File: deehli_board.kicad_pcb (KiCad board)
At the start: 2 copper layers, 84 x 51 mm, 46 parts, among them J1 Servo_Out, J2 PWM_In, J3 Vcc_Out, J4 ZDT_Pins, J5 CAN_Ext, J6 Board_IO, J7 ZDT_Connector, SW1 SW_DPDT_x2, U1 APE1707M-50-HF, U2 LM2576HVT-5, U3 LM2576HVT-5, U4 LM2576HVT-15, U5 LD1117S33TR_SOT223, U6 LM2576HVT-15

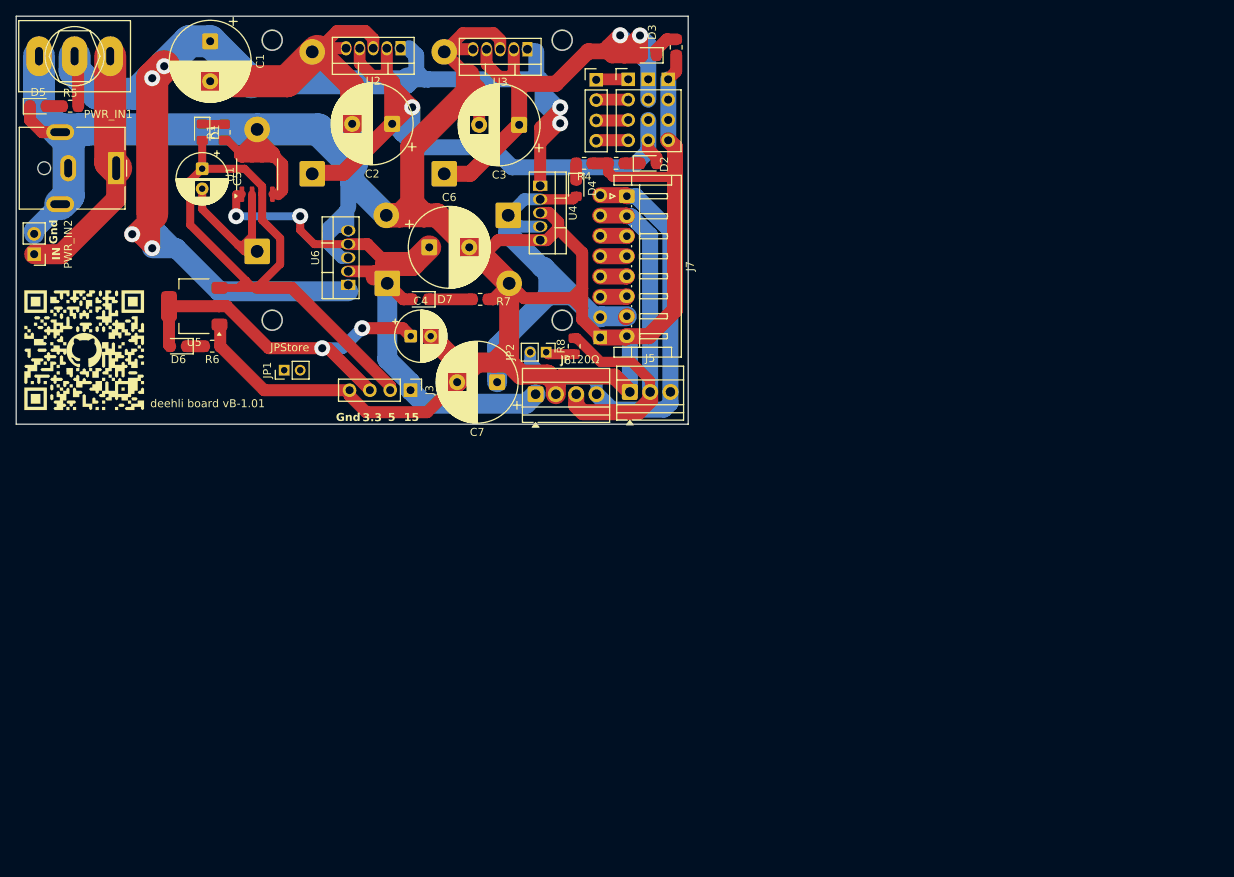
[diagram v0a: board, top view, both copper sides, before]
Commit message: VB-1.02
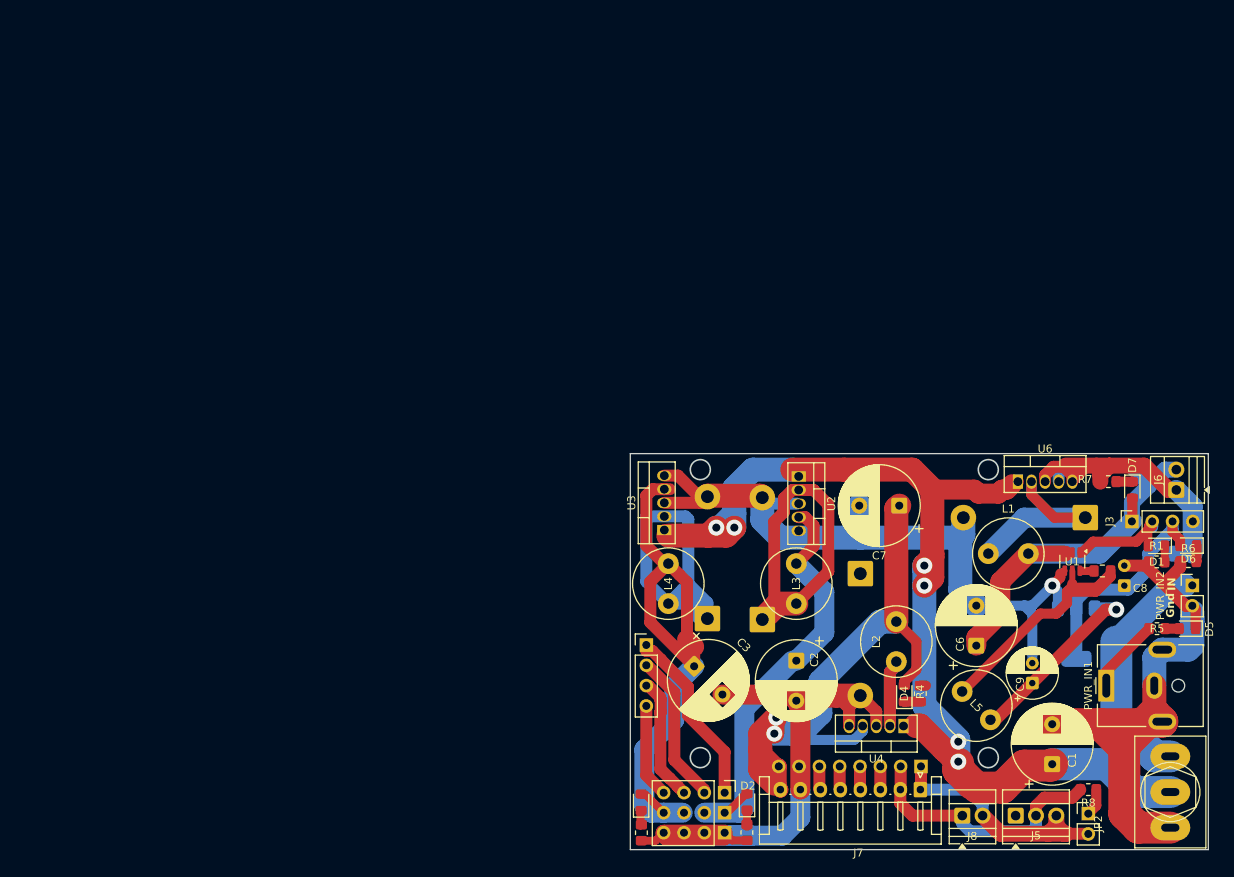
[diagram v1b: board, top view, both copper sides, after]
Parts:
- removed C5: Cpol 200uF, Capacitor_THT:CP_Radial_D6.3mm_P2.50mm
- removed D12: 1N5822, Diode_THT:D_DO-201AD_P15.24mm_Horizontal
- removed JP1: Jumper_Dummy, Connector_PinHeader_2.00mm:PinHeader_1x02_P2.00mm_Vertical
- added C8: 100nF, Capacitor_SMD:C_0805_2012Metric_Pad1.18x1.45mm_HandSolder, F.Cu at (163.8, 105.3)
- added C9: Cpol 2x22uF, Capacitor_THT:CP_Radial_D6.3mm_P2.50mm, F.Cu at (155.0, 119.4)
- added J8: BoardCAN, TerminalBlock:TerminalBlock_Xinya_XY308-2.54-2P_1x02_P2.54mm_Horizontal, F.Cu at (146.3, 135.9)
- added L1: 100u, Inductor_THT:L_Radial_D8.7mm_P5.00mm_Fastron_07HCP, F.Cu at (149.5, 103.2)
- added L2: 100u, Inductor_THT:L_Radial_D8.7mm_P5.00mm_Fastron_07HCP, F.Cu at (138.0, 116.7)
- added L3: 100u, Inductor_THT:L_Radial_D8.7mm_P5.00mm_Fastron_07HCP, F.Cu at (125.5, 109.4)
- added L4: 100u, Inductor_THT:L_Radial_D8.7mm_P5.00mm_Fastron_07HCP, F.Cu at (109.5, 109.4)
- added L5: 4.7u, Inductor_THT:L_Radial_D8.7mm_P5.00mm_Fastron_07HCP, F.Cu at (146.2, 120.4)
- C4, G***, U5: moved to B.Cu
- J3: footprint Connector_PinHeader_2.54mm:PinHeader_1x04_P2.54mm_Vertical -> Connector_PinSocket_2.54mm:PinSocket_1x04_P2.54mm_Vertical
- J4: footprint Connector_PinHeader_2.54mm:PinHeader_1x08_P2.54mm_Horizontal -> Connector_PinSocket_2.54mm:PinSocket_1x08_P2.54mm_Horizontal
- J6: value Board_IO -> BoardPWR; footprint TerminalBlock:TerminalBlock_Xinya_XY308-2.54-4P_1x04_P2.54mm_Horizontal -> TerminalBlock:TerminalBlock_Xinya_XY308-2.54-2P_1x02_P2.54mm_Horizontal
- JP2: footprint Connector_PinHeader_2.00mm:PinHeader_1x02_P2.00mm_Vertical -> Connector_PinHeader_2.54mm:PinHeader_1x02_P2.54mm_Vertical
- R5: value 15k -> 50k
- U1: value APE1707M-50-HF -> AP63205WU; footprint Package_SO:SOIC-8_3.9x4.9mm_P1.27mm -> Package_TO_SOT_SMD:TSOT-23-6
- moved SW1 165.0 mm to (172.3, 133.0), turned to 90 degrees
- moved D5 157.8 mm to (174.4, 112.6), turned to 180 degrees
- moved R5 150.7 mm to (170.6, 112.6), turned to 180 degrees
- moved PWR_IN2 150.6 mm to (175.0, 107.2), turned to 0 degrees
- moved PWR_IN1 139.6 mm to (164.3, 119.7), turned to 90 degrees
- moved C1 138.7 mm to (157.5, 129.5), turned to 90 degrees
- moved G*** 137.4 mm to (164.0, 129.0), turned to 180 degrees
- moved D1 130.0 mm to (170.5, 102.2), turned to 180 degrees
- moved D6 128.7 mm to (174.5, 102.2)
- moved R1 128.3 mm to (170.6, 104.2), turned to 0 degrees
- moved R6 124.9 mm to (174.5, 104.2), turned to 0 degrees
- moved U5 117.6 mm to (160.5, 113.2), turned to -90 degrees
- moved U1 112.8 mm to (160.0, 104.2), turned to -90 degrees
- moved R2 98.3 mm to (106.1, 138.1)
- moved C4 94.5 mm to (166.5, 107.2), turned to 90 degrees
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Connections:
- D10 pad 1: 5V_Servo12 -> Net-(D10-K)
- D11 pad 1: 15V_Other -> Net-(D11-K)
- D8 pad 1: 15V_ZDT -> Net-(D8-K)
- D9 pad 1: 5V_Servo34 -> Net-(D9-K)
- J1 pad 5: 5V_Servo12 -> 5V_Servo34
- J1 pad 6: 5V_Servo12 -> 5V_Servo34
- J1 pad 7: 5V_Servo34 -> 5V_Servo12
- J1 pad 8: 5V_Servo34 -> 5V_Servo12
- J4 pad 1: GND -> CAN_L
- J4 pad 2: 15V_ZDT -> CAN_H
- J4 pad 7: CAN_H -> GND
- J4 pad 8: CAN_L -> 15V_ZDT
- J6 pad 1: 15V_Other -> GND
- J6 pad 2: GND -> 15V_Other
- J7 pad 3: Net-(J4-Pin_6) -> Net-(J4-Pin_3)
- J7 pad 4: Net-(J4-Pin_5) -> Net-(J4-Pin_4)
- J7 pad 5: Net-(J4-Pin_4) -> Net-(J4-Pin_5)
- J7 pad 6: Net-(J4-Pin_3) -> Net-(J4-Pin_6)
- J7 pad 7: 15V_ZDT -> GND
- J7 pad 8: GND -> 15V_ZDT
- R5 pad 2: Net-(SW1A-B) -> Net-(PWR_IN2-Pin_1)
- U1 pad 1: 15V_Other -> 5V_Other
- U1 pad 2: Net-(D12-K) -> 15V_Other
- U1 pad 3: 5V_Other -> 15V_Other
- U1 pad 5: GND -> Net-(U1-SW)
- U1 pad 6: GND -> Net-(U1-BST)
- U2 pad 2: 5V_Servo34 -> Net-(D9-K)
- U3 pad 2: 5V_Servo12 -> Net-(D10-K)
- U4 pad 2: 15V_ZDT -> Net-(D8-K)
- U6 pad 2: 15V_Other -> Net-(D11-K)
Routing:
- net GND: track 428.8 -> 316.1 mm, vias 0 -> 1
- net Net-(D10-K): track 0.00 -> 45.8 mm
- net Net-(D9-K): track 0.00 -> 42.1 mm
- net 5V_Other: track 73.8 -> 38.8 mm, vias 0 -> 1
- net Net-(U1-SW): track 0.00 -> 34.6 mm
- net 5V_Servo34: track 86.3 -> 52.8 mm, vias 1 -> 0
- net Net-(D11-K): track 0.00 -> 33.1 mm
- net Net-(SW1A-B): track 173.7 -> 146.7 mm
- net CAN_L: track 54.6 -> 31.4 mm
- net 15V_ZDT: track 56.9 -> 79.5 mm, vias 0 -> 2
- net Net-(D12-K): track 21.3 -> 0.00 mm
- net CAN_H: track 52.6 -> 32.9 mm
- net Net-(J1-Pin_1): track 4.03 -> 23.0 mm
- net 3.3V_Other: track 47.0 -> 28.6 mm, vias 2 -> 0
- net 15V_Other: track 77.6 -> 60.0 mm, vias 2 -> 0
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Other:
- board size 84 x 51 mm -> 72.2 x 49.5 mm
- board text added: "deehli board vB-1.02"
- board text removed: "15"
- board text removed: "3.3"
- board text removed: "5"
- board text removed: "JP120Ω"
- board text removed: "JPStore"
- board text removed: "deehli board vB-1.01"
